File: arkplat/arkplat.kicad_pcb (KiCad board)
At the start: 2 copper layers, 1 part, among them U1 portenta

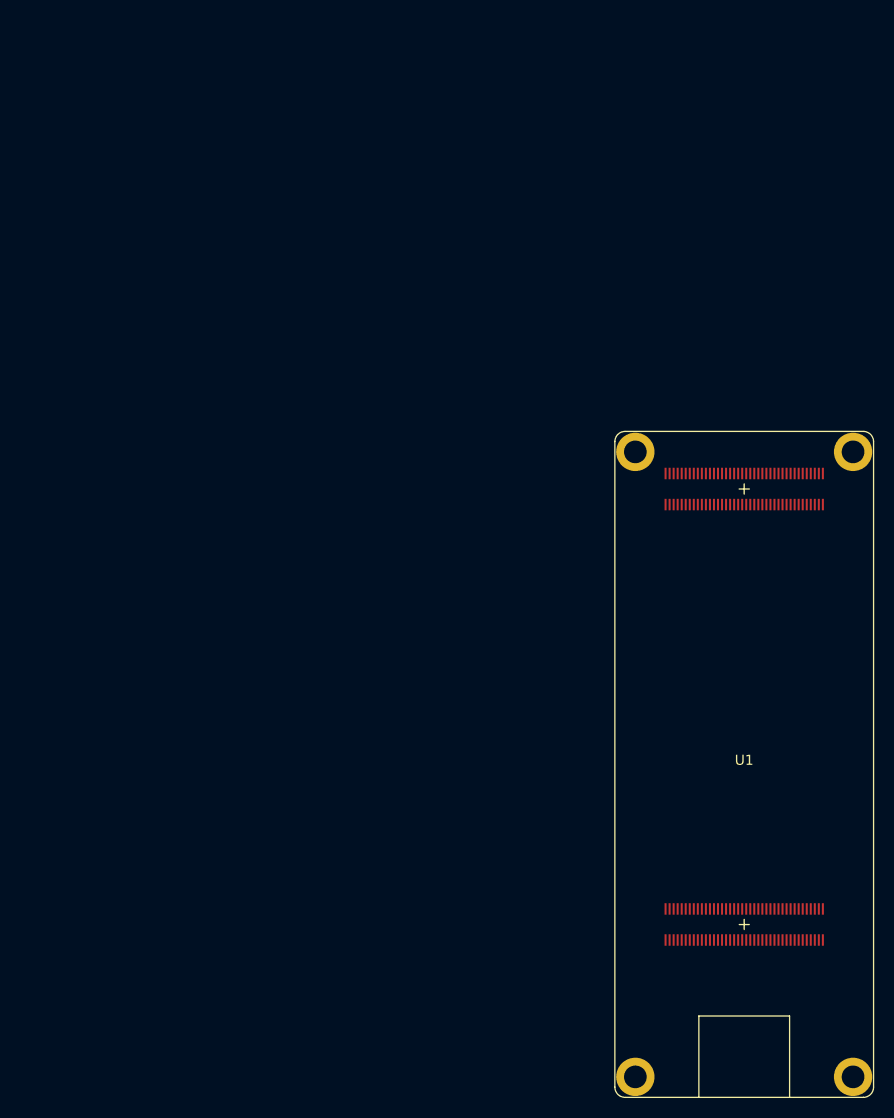
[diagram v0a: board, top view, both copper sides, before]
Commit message: wip on poe
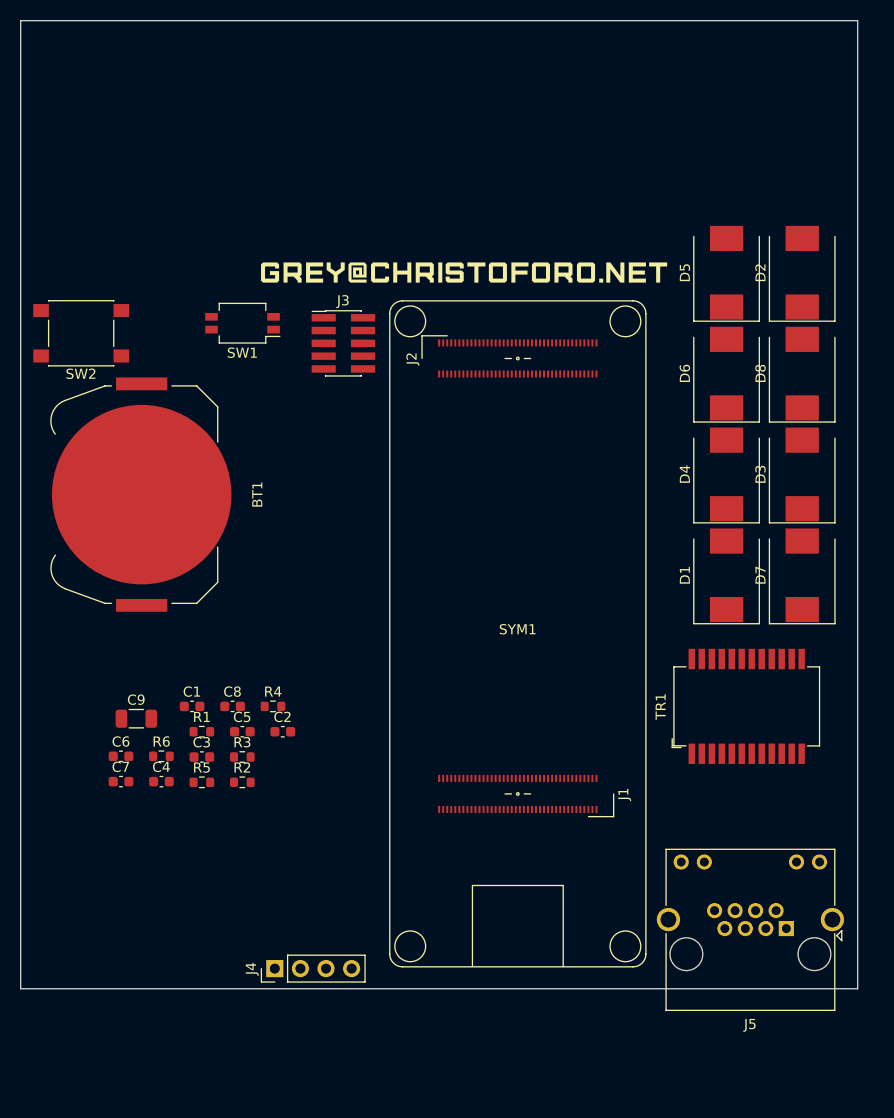
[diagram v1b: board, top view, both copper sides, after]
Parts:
- removed U1: portenta, custom_footprints:portenta
- added BT1: Battery_Cell, Battery:BatteryHolder_Keystone_3034_1x20mm, F.Cu at (77.0, 77.0)
- added C1: 100nF, Capacitor_SMD:C_0603_1608Metric, F.Cu at (82.0, 98.0)
- added C2: 100nF, Capacitor_SMD:C_0603_1608Metric, F.Cu at (91.0, 100.5)
- added C3: 100nF, Capacitor_SMD:C_0603_1608Metric, F.Cu at (83.0, 103.0)
- added C4: 100nF, Capacitor_SMD:C_0603_1608Metric, F.Cu at (79.0, 105.5)
- added C5: 0.039uF, Capacitor_SMD:C_0603_1608Metric, F.Cu at (87.0, 100.5)
- added C6: 0.039uF, Capacitor_SMD:C_0603_1608Metric, F.Cu at (75.0, 103.0)
- added C7: 0.039uF, Capacitor_SMD:C_0603_1608Metric, F.Cu at (75.0, 105.5)
- added C8: 0.039uF, Capacitor_SMD:C_0603_1608Metric, F.Cu at (86.0, 98.0)
- added C9: 1000pF, Capacitor_SMD:C_1206_3216Metric, F.Cu at (76.5, 99.2)
- added D1: D_Schottky, Diode_SMD:D_SMC, F.Cu at (135.0, 85.0)
- added D2: D_Schottky, Diode_SMD:D_SMC, F.Cu at (142.5, 55.0)
- added D3: D_Schottky, Diode_SMD:D_SMC, F.Cu at (142.5, 75.0)
- added D4: D_Schottky, Diode_SMD:D_SMC, F.Cu at (135.0, 75.0)
- added D5: D_Schottky, Diode_SMD:D_SMC, F.Cu at (135.0, 55.0)
- added D6: D_Schottky, Diode_SMD:D_SMC, F.Cu at (135.0, 65.0)
- added D7: D_Schottky, Diode_SMD:D_SMC, F.Cu at (142.5, 85.0)
- added D8: D_Schottky, Diode_SMD:D_SMC, F.Cu at (142.5, 65.0)
- added J1: portenta_HD_J1, custom_footprints:DF40HC(3.5)-80DS-0.4V(51), F.Cu at (114.3, 106.7)
- added J2: portenta_HD_J2, custom_footprints:DF40HC(3.5)-80DS-0.4V(51), F.Cu at (114.3, 63.5)
- added J3: Conn_02x05_Odd_Even, Connector_PinHeader_1.27mm:PinHeader_2x05_P1.27mm_Vertical_SMD, F.Cu at (97.0, 62.0)
- added J4: Conn_01x04, Connector_PinHeader_2.54mm:PinHeader_1x04_P2.54mm_Vertical, F.Cu at (90.2, 124.0)
- added J5: RJ45_LED_Shielded, Connector_RJ:RJ45_Amphenol_RJHSE538X, F.Cu at (140.9, 120.0)
- added LOGO1: Logo_Open_Hardware_Small, custom_footprints:logo, F.Cu at (109.0, 55.0)
- added LOGO2: Logo_Open_Hardware_Small, custom_footprints:logo, B.Cu at (109.0, 55.0)
- added R1: 470, Resistor_SMD:R_0603_1608Metric, F.Cu at (83.0, 100.5)
- added R2: 470, Resistor_SMD:R_0603_1608Metric, F.Cu at (87.0, 105.5)
- added R3: 75, Resistor_SMD:R_0603_1608Metric, F.Cu at (87.0, 103.0)
- added R4: 75, Resistor_SMD:R_0603_1608Metric, F.Cu at (90.0, 98.0)
- added R5: 75, Resistor_SMD:R_0603_1608Metric, F.Cu at (83.0, 105.5)
- added R6: 75, Resistor_SMD:R_0603_1608Metric, F.Cu at (79.0, 103.0)
- added SW1: SW_DIP_x02, Button_Switch_SMD:SW_DIP_SPSTx02_Slide_Omron_A6H-2101_W6.15mm_P1.27mm, F.Cu at (87.0, 60.0)
- added SW2: SW_Push, Button_Switch_SMD:SW_SPST_PTS645, F.Cu at (71.0, 61.0)
- added SYM1: SYM_Flash_Small, custom_footprints:portenta, F.Cu at (114.3, 106.7)
- added TR1: TG111-MSC13LF, Transformer_SMD:Transformer_Ethernet_HALO_TG111-MSC13, F.Cu at (137.0, 98.0)
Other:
- board outline added: 83 x 96 mm
